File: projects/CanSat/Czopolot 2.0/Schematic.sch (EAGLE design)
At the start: 112 parts

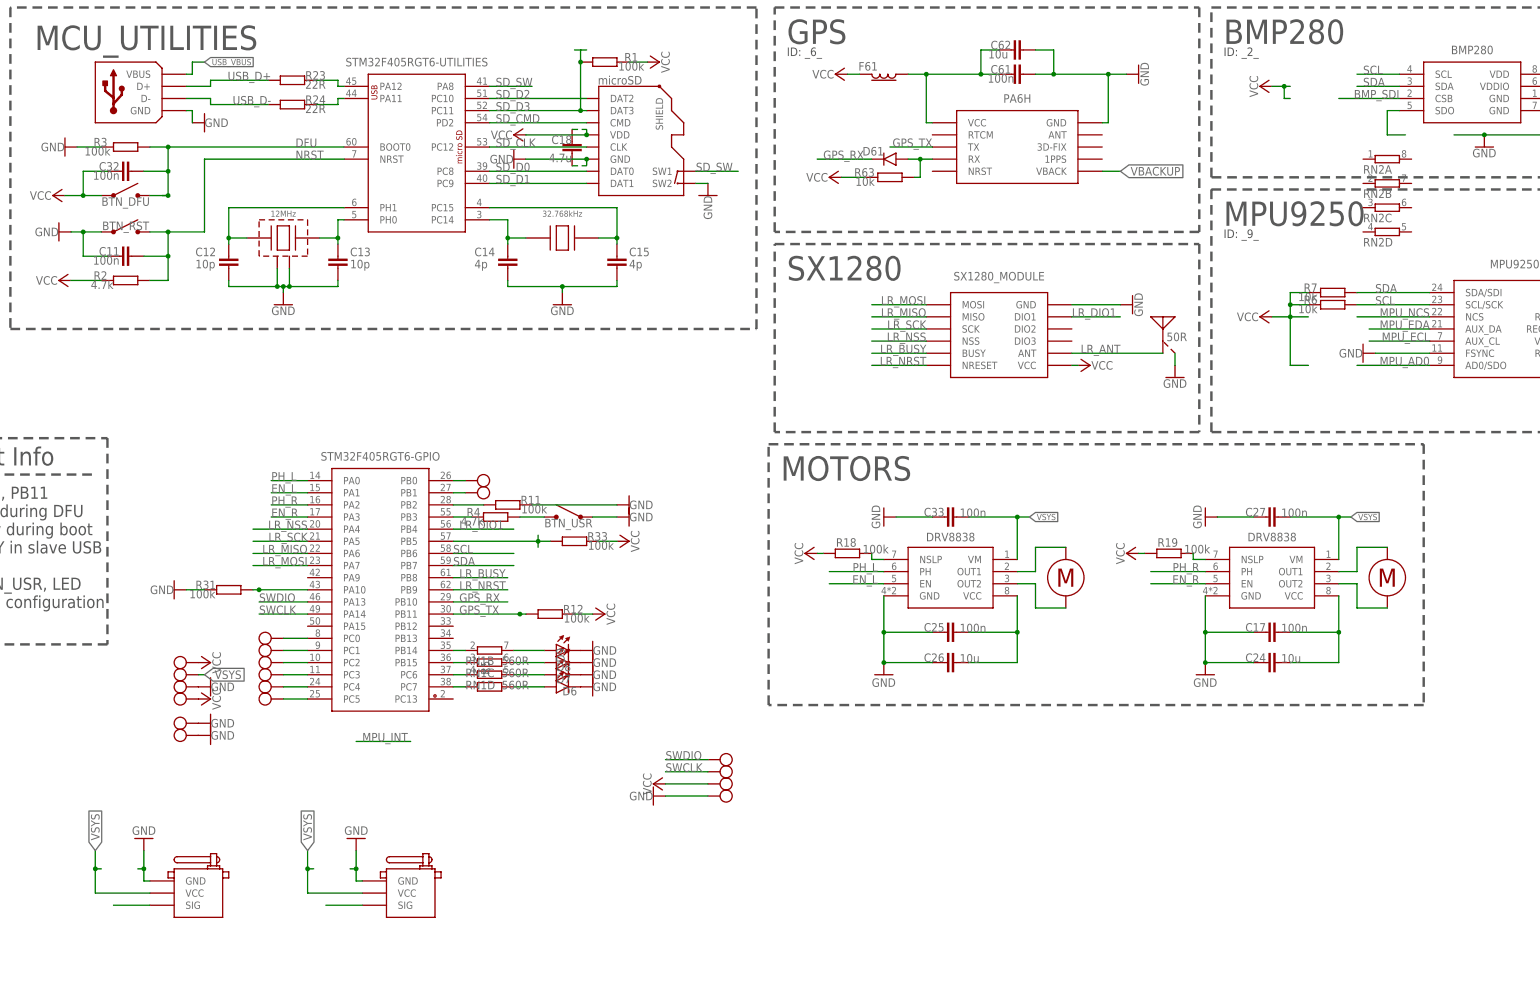
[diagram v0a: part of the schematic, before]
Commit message: Pads backup
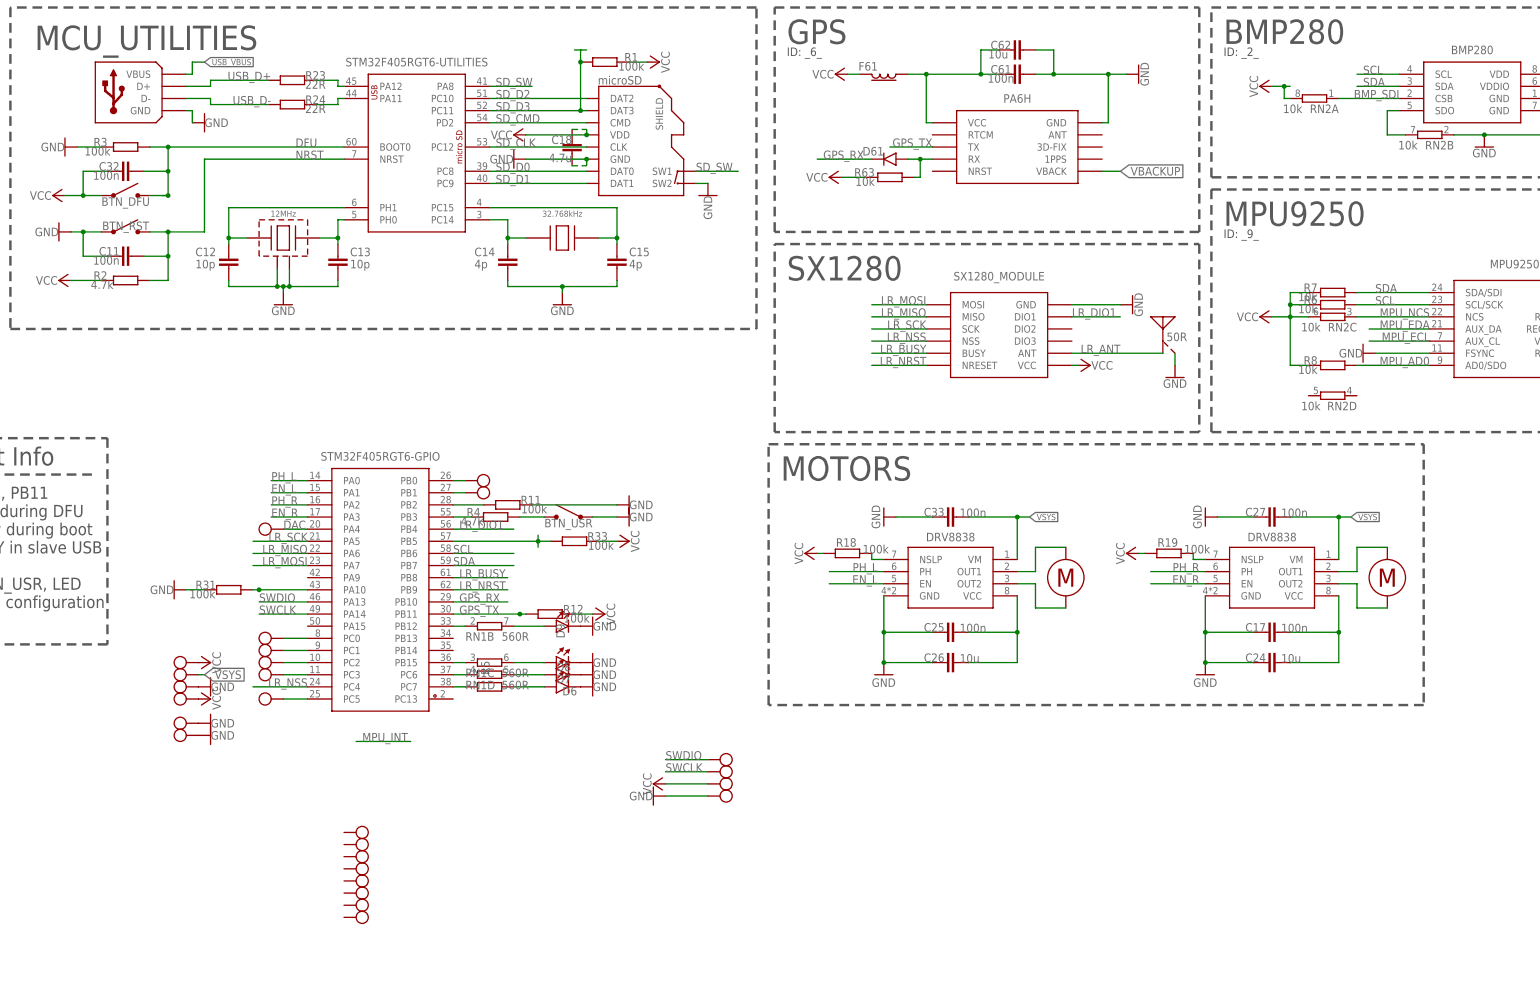
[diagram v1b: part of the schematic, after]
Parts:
- removed U$16: SERVO, Unified:SERVO
- added R8: 10k, Unified:RESISTOR0603
- RN2: value (none) -> 10k
- U$13: value SERVO -> GPIO_PADS; device Unified:SERVO -> SobieskiSat2:GPIO_PADS
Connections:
- removed net N$41: U$13.SIG
- removed net N$42: U$16.SIG
- removed net N$49: U$1STM32F405RGT6_GPIO.PC4, U$27.1
- new net DAC: U$1STM32F405RGT6_GPIO.PA4, U$27.1
- net BMP_SDI: now also RN2A.1
- net BMP_SDO: now also RN2B.2
- net GND: now also RN2B.1; no longer U$13.GND, U$16.GND
- net LR_NSS: now also U$1STM32F405RGT6_GPIO.PC4; no longer U$1STM32F405RGT6_GPIO.PA4
- net MPU_AD0: now also R8.1
- net MPU_NCS: now also RN2C.1
- net N$28: now also U$1STM32F405RGT6_GPIO.PB12; no longer U$1STM32F405RGT6_GPIO.PB14
- net VCC: now also R8.2, RN2A.2, RN2C.2
- net VSYS: no longer U$13.VCC, U$16.VCC
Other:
- moved on the sheet: D9, RN1B, RN2A, RN2B, RN2C, RN2D
